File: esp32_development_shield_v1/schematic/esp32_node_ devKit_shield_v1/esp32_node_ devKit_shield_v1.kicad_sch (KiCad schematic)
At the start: 37 parts, among them J1 Screw_Terminal_01x02, J10 Screw_Terminal_01x02, J11 Screw_Terminal_01x02, J12 Screw_Terminal_01x02, J13 Screw_Terminal_01x02, J14 Screw_Terminal_01x02, J15 Screw_Terminal_01x02, J16 Screw_Terminal_01x02, J17 Screw_Terminal_01x02, J19 Screw_Terminal_01x02, J2 Conn_02x20_Odd_Even, J20 Screw_Terminal_01x02, J21 Screw_Terminal_01x02, J22 Screw_Terminal_01x02, J23 Screw_Terminal_01x02, J24 Screw_Terminal_01x02, J25 Screw_Terminal_01x02, J26 Screw_Terminal_01x02, J27 Conn_01x04, J28 Conn_01x04, J29 Conn_01x04, J3 Conn_02x20_Odd_Even, J30 Conn_01x04, J31 USB_C_Receptacle_PowerOnly_6P, J4 Conn_01x04, J5 Conn_01x04, J6 Conn_01x04, J7 Conn_01x04, J8 Screw_Terminal_01x02, J9 Screw_Terminal_01x02, U2 AMS1117-3.3

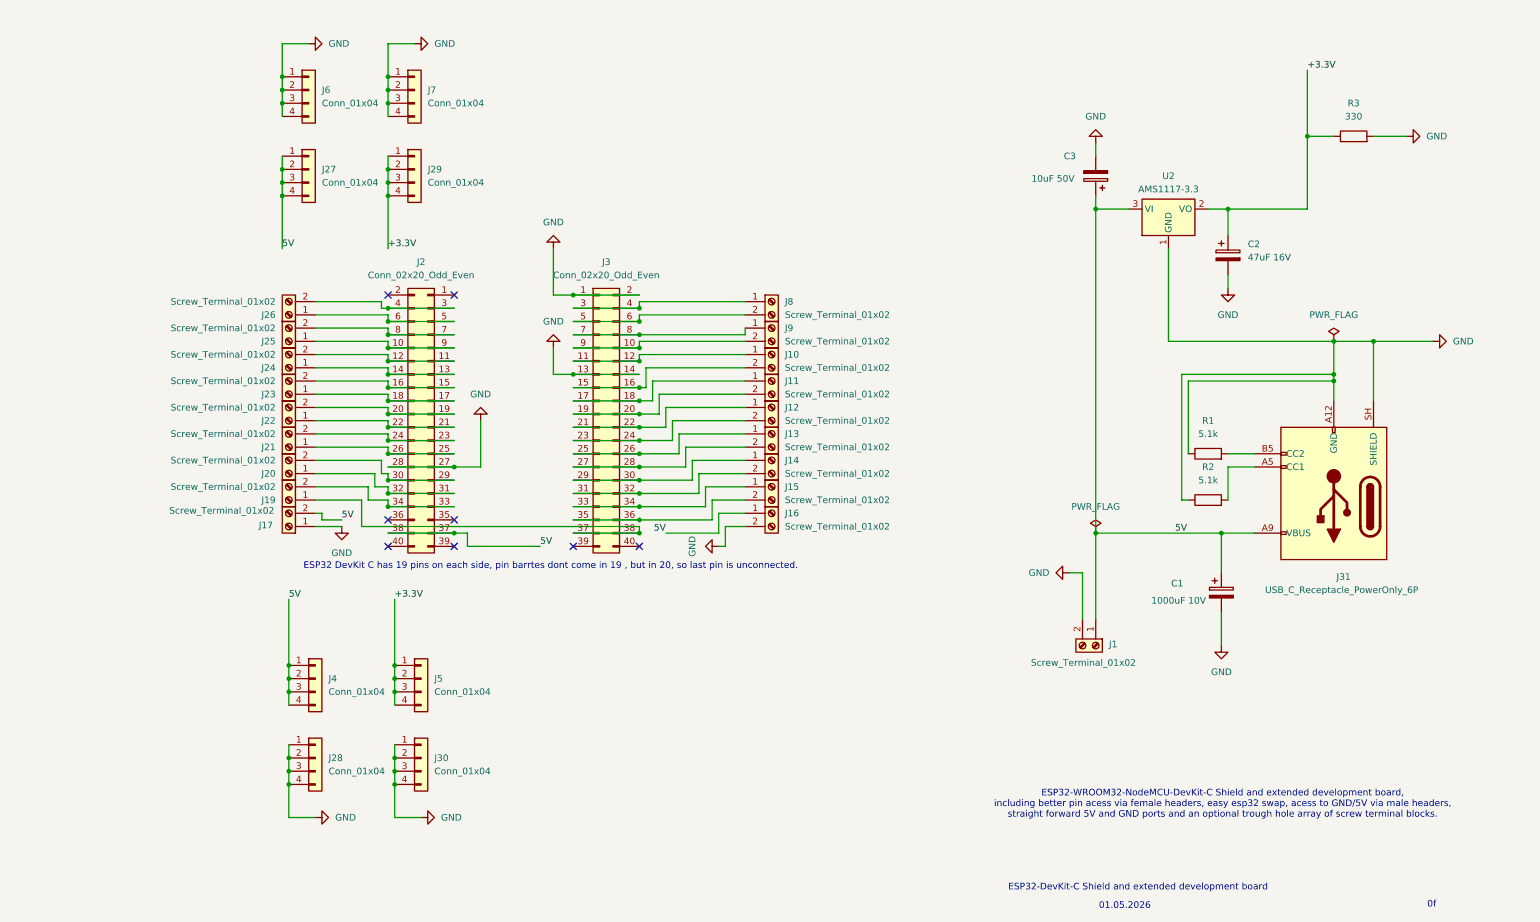
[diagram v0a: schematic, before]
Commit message: *
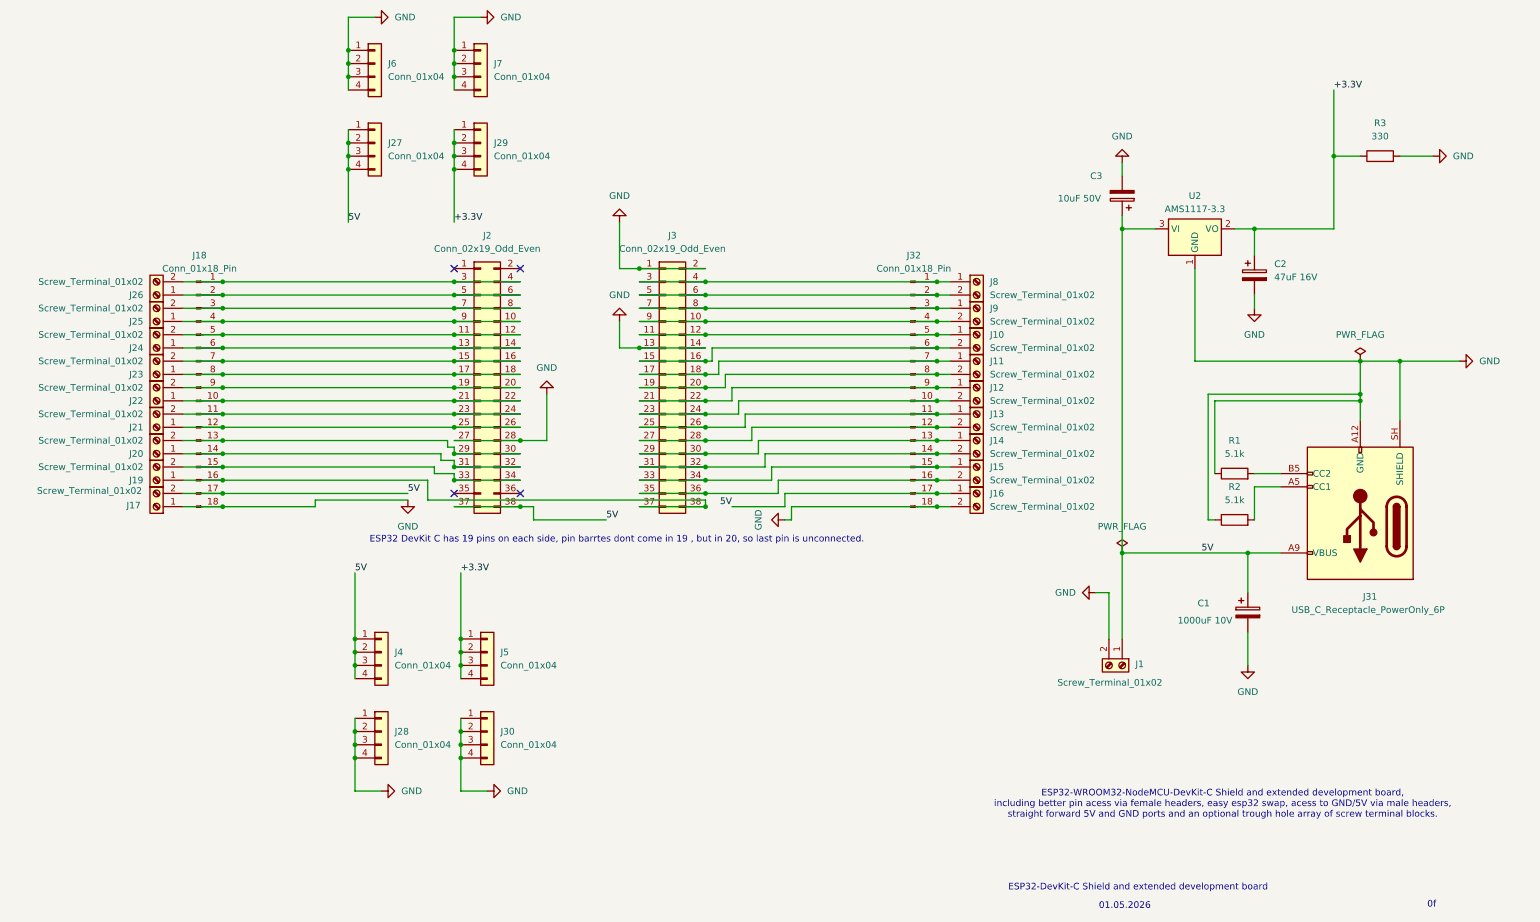
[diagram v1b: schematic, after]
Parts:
- removed J2, J3: Conn_02x20_Odd_Even, Connector_PinSocket_2.54mm:PinSocket_2x20_P2.54mm_Vertical, symbol Connector_Generic:Conn_02x20_Odd_Even
- added J18, J32: Conn_01x18_Pin, Connector_PinSocket_2.54mm:PinSocket_1x18_P2.54mm_Vertical, symbol Connector:Conn_01x18_Pin
- added J2, J3: Conn_02x19_Odd_Even, Connector_PinSocket_2.54mm:PinSocket_2x19_P2.54mm_Vertical, symbol Connector_Generic:Conn_02x19_Odd_Even
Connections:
- net 5V: now also J18.17 (Pin_17), J2.37 (Pin_37), J2.38 (Pin_38), J32.17 (Pin_17)
- net GND: now also J18.18 (Pin_18), J2.27 (Pin_27), J2.28 (Pin_28), J3.1 (Pin_1), J3.13 (Pin_13), J3.14 (Pin_14), J3.2 (Pin_2), J32.18 (Pin_18)
- net at J21.1 (Pin_1): now also J18.12 (Pin_12), J2.25 (Pin_25), J2.26 (Pin_26)
- net at J21.2 (Pin_2): now also J18.11 (Pin_11), J2.23 (Pin_23), J2.24 (Pin_24)
- net at J13.1 (Pin_1): now also J3.25 (Pin_25), J3.26 (Pin_26), J32.11 (Pin_11)
- net at J13.2 (Pin_2): now also J3.27 (Pin_27), J3.28 (Pin_28), J32.12 (Pin_12)
- net at J20.1 (Pin_1): now also J18.14 (Pin_14), J2.31 (Pin_31), J2.32 (Pin_32)
- net at J20.2 (Pin_2): now also J18.13 (Pin_13), J2.29 (Pin_29), J2.30 (Pin_30)
- net at J12.1 (Pin_1): now also J3.21 (Pin_21), J3.22 (Pin_22), J32.9 (Pin_9)
- net at J12.2 (Pin_2): now also J3.23 (Pin_23), J3.24 (Pin_24), J32.10 (Pin_10)
- net at J15.1 (Pin_1): now also J3.33 (Pin_33), J3.34 (Pin_34), J32.15 (Pin_15)
- net at J15.2 (Pin_2): now also J3.35 (Pin_35), J3.36 (Pin_36), J32.16 (Pin_16)
- net at J24.1 (Pin_1): now also J18.6 (Pin_6), J2.13 (Pin_13), J2.14 (Pin_14)
- net at J24.2 (Pin_2): now also J18.5 (Pin_5), J2.11 (Pin_11), J2.12 (Pin_12)
- net at J9.1 (Pin_1): now also J3.7 (Pin_7), J3.8 (Pin_8), J32.3 (Pin_3)
- net at J9.2 (Pin_2): now also J3.10 (Pin_10), J3.9 (Pin_9), J32.4 (Pin_4)
- net at J19.1 (Pin_1): now also J18.16 (Pin_16), J3.37 (Pin_37), J3.38 (Pin_38)
- net at J19.2 (Pin_2): now also J18.15 (Pin_15), J2.33 (Pin_33), J2.34 (Pin_34)
- net at J8.1 (Pin_1): now also J3.3 (Pin_3), J3.4 (Pin_4), J32.1 (Pin_1)
- net at J8.2 (Pin_2): now also J3.5 (Pin_5), J3.6 (Pin_6), J32.2 (Pin_2)
- net at J23.1 (Pin_1): now also J18.8 (Pin_8), J2.17 (Pin_17), J2.18 (Pin_18)
- net at J23.2 (Pin_2): now also J18.7 (Pin_7), J2.15 (Pin_15), J2.16 (Pin_16)
- net at J25.1 (Pin_1): now also J18.4 (Pin_4), J2.10 (Pin_10), J2.9 (Pin_9)
- net at J25.2 (Pin_2): now also J18.3 (Pin_3), J2.7 (Pin_7), J2.8 (Pin_8)
- net at J22.2 (Pin_2): now also J18.9 (Pin_9), J2.19 (Pin_19), J2.20 (Pin_20)
- net at J22.1 (Pin_1): now also J18.10 (Pin_10), J2.21 (Pin_21), J2.22 (Pin_22)
- net at J26.2 (Pin_2): now also J18.1 (Pin_1), J2.3 (Pin_3), J2.4 (Pin_4)
- net at J26.1 (Pin_1): now also J18.2 (Pin_2), J2.5 (Pin_5), J2.6 (Pin_6)
- net at J11.1 (Pin_1): now also J3.17 (Pin_17), J3.18 (Pin_18), J32.7 (Pin_7)
- net at J11.2 (Pin_2): now also J3.19 (Pin_19), J3.20 (Pin_20), J32.8 (Pin_8)
- net at J14.1 (Pin_1): now also J3.29 (Pin_29), J3.30 (Pin_30), J32.13 (Pin_13)
- net at J14.2 (Pin_2): now also J3.31 (Pin_31), J3.32 (Pin_32), J32.14 (Pin_14)
- net at J10.1 (Pin_1): now also J3.11 (Pin_11), J3.12 (Pin_12), J32.5 (Pin_5)
- net at J10.2 (Pin_2): now also J3.15 (Pin_15), J3.16 (Pin_16), J32.6 (Pin_6)
- no-connect marks 8 -> 4
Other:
- moved on the sheet: C1, C2, C3, J1, J10, J11, J12, J13, J14, J15, J16, J17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
